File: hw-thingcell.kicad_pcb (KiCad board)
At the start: 2 copper layers, 32.5 x 67 mm, 99 parts, among them J1 Conn_01x02_Pin, J2 Conn_01x08_Pin, J3 USB4510-03-1-A, J4 Conn_01x08_Pin, J5 GSM_ANT, J6 GNSS_ANT, J7 SIM8060-6-0-14-00-A, Q1 PMBT3904235, Q2 PMBT3904235, Q3 PMBT3904235, U1 AP62301WU-7, U2 AP62301WU-7, U3 ESP32-S2-SOLO, U4 SIM868, U5 CH340C, Y1 32.768k

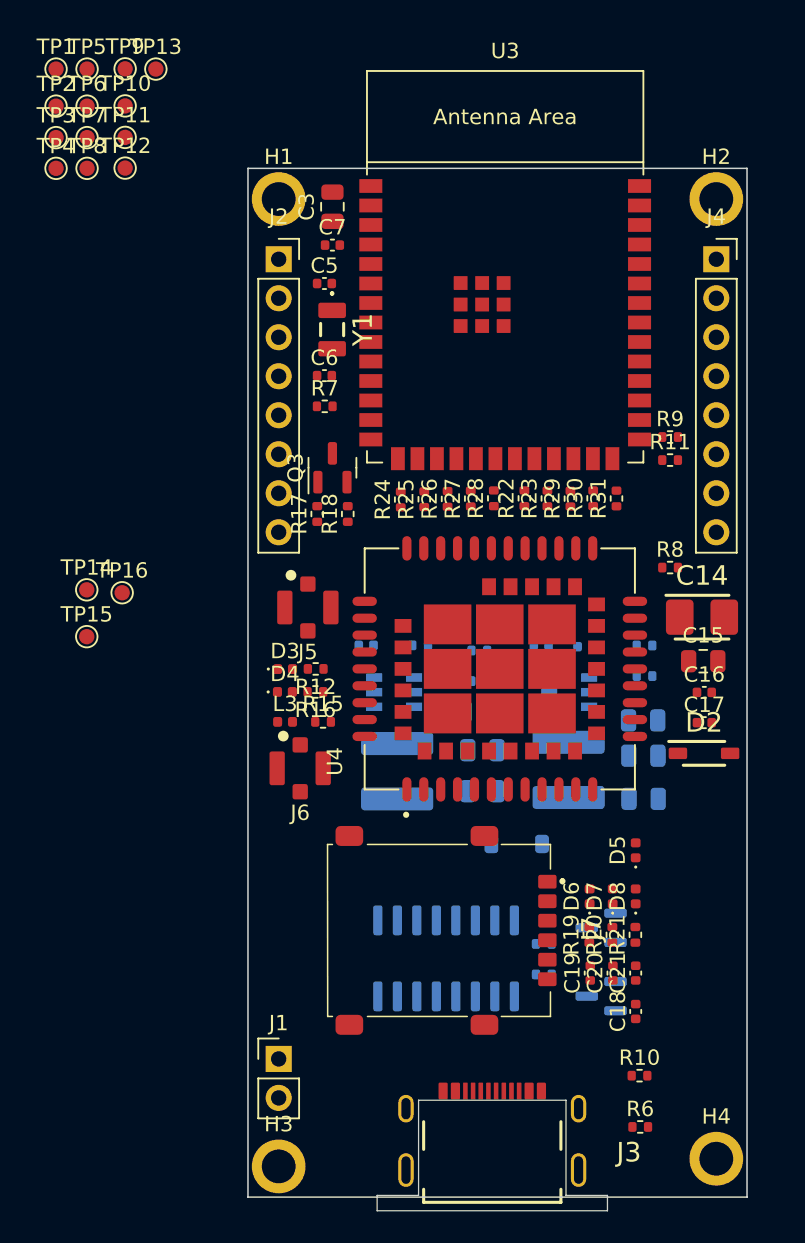
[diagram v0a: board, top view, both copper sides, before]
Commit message: First placement
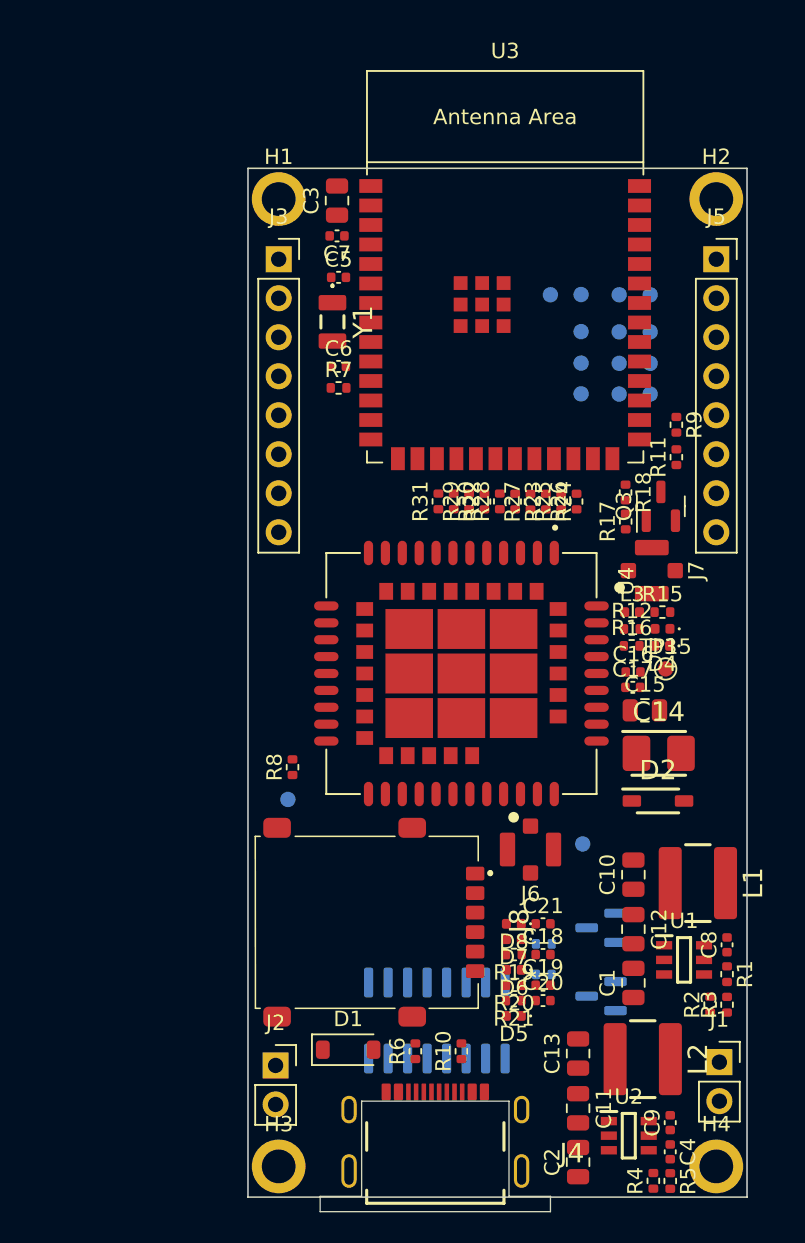
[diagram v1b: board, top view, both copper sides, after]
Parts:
- added J1: Conn_01x02_Pin, Connector_PinSocket_2.54mm:PinSocket_1x02_P2.54mm_Vertical, F.Cu at (151.7, 125.2)
- C1, C10, C11, C12, C13, C2, C4, C8, C9, D1, L1, L2, R1, R2, R3, R4, R5, U1, U2: moved to F.Cu
- J2: renamed from J1; footprint Connector_PinHeader_2.54mm:PinHeader_1x02_P2.54mm_Vertical -> Connector_PinSocket_2.54mm:PinSocket_1x02_P2.54mm_Vertical
- TP1, TP10, TP11, TP12, TP13, TP14, TP16, TP2, TP3, TP4, TP5, TP6, TP7, TP8, TP9: moved to B.Cu
- moved TP1 41.4 mm to (147.2, 75.2), turned to 180 degrees
- moved TP2 41.4 mm to (147.2, 77.7), turned to 180 degrees
- moved TP3 41.4 mm to (147.2, 79.7), turned to 180 degrees
- moved TP4 41.4 mm to (147.2, 81.7), turned to 180 degrees
- moved TP15 37.8 mm to (148.2, 99.6)
- moved TP5 37.6 mm to (145.2, 75.2), turned to 180 degrees
- moved TP6 37.6 mm to (145.2, 77.7), turned to 180 degrees
- moved TP7 37.6 mm to (145.2, 79.7), turned to 180 degrees
- moved TP8 37.6 mm to (145.2, 81.7), turned to 180 degrees
- moved R4 34.9 mm to (147.4, 132.9), turned to 90 degrees
- moved TP16 34.2 mm to (142.8, 111.0), turned to 180 degrees
- moved C4 33.4 mm to (148.5, 131.1), turned to -90 degrees
- moved TP10 33.1 mm to (142.7, 77.6), turned to 180 degrees
- moved TP11 33.1 mm to (142.7, 79.7), turned to 180 degrees
- moved TP12 33.1 mm to (142.7, 81.7), turned to 180 degrees
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- renumbered J2 to J3, J3 to J4, J4 to J5, J5 to J6, J6 to J7, J7 to J8

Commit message: Routed all components
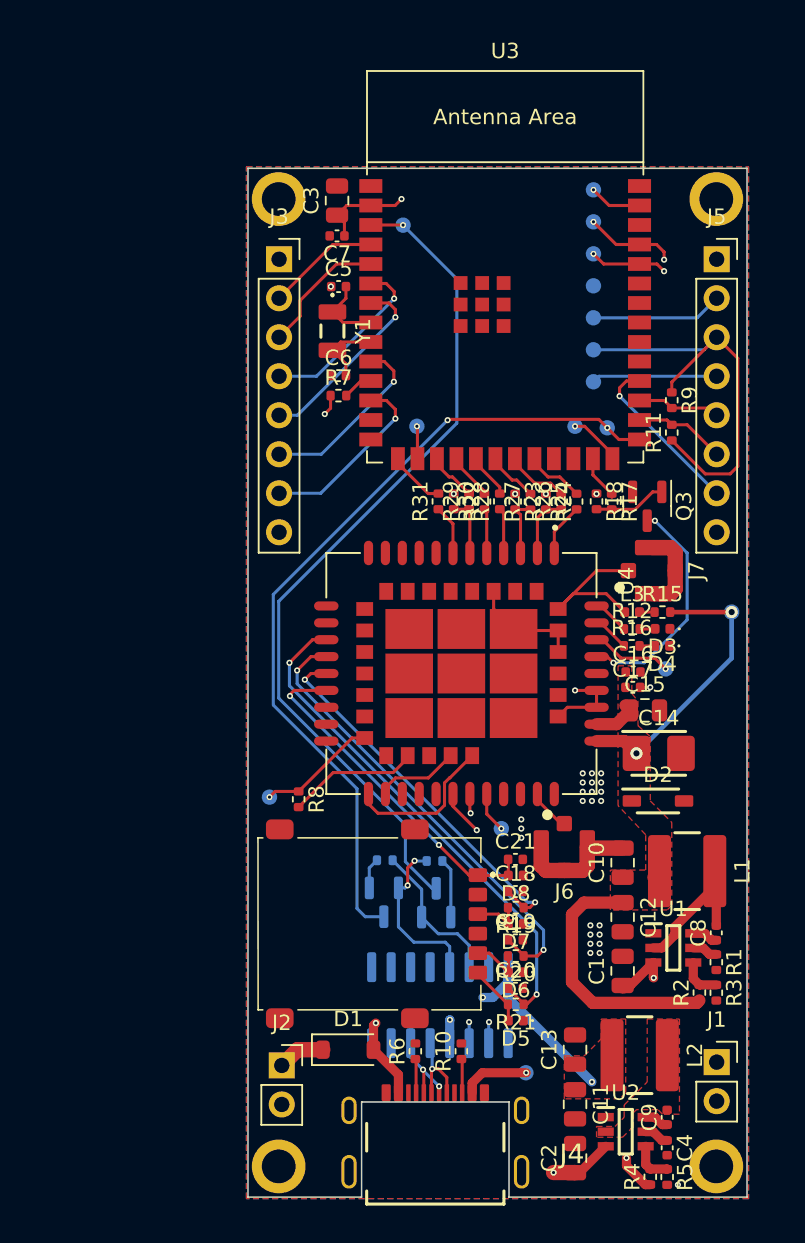
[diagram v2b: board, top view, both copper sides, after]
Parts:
- TP15: moved to B.Cu
- moved TP4 44.9 mm to (139.1, 125.9)
- moved TP3 17.0 mm to (152.5, 95.9)
- moved TP7 16.7 mm to (131.1, 70.7)
- moved Q2 15.4 mm to (129.8, 114.8), turned to -90 degrees
- moved TP8 13.3 mm to (132.0, 83.8)
- moved R14 12.7 mm to (129.9, 112.1), turned to 0 degrees
- moved Q1 10.9 mm to (133.3, 114.8), turned to 90 degrees
- moved TP11 9.24 mm to (143.5, 70.5)
- moved R13 8.93 mm to (133.2, 112.1)
- moved TP9 8.59 mm to (142.3, 83.8)
- moved TP13 7.39 mm to (143.5, 68.4)
- moved TP16 5.39 mm to (137.5, 110.0)
- moved TP10 5.13 mm to (143.5, 72.6)
- moved C21 4.56 mm to (138.4, 112.0)
- moved C18 4.48 mm to (138.4, 114.1)
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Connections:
- U3 pad 10: /D6/MOSI -> /D8
- U3 pad 12: /ESP_IO34 -> /D9/S_DET
- U3 pad 15: /ESP_RTS -> /ESP_IO34
- U3 pad 17: /PK_CTL -> /ESP_IO32
- U3 pad 18: /D1/SCL -> /ESP_IO33
- U3 pad 19: /D2/SDA -> /ESP_CTS
- U3 pad 20: /D3 -> /ESP_RTS
- U3 pad 21: /D4/SCK -> /ESP_TXD
- U3 pad 22: /D5/MISO -> /ESP_RXD
- U3 pad 24: /D7/SS -> unconnected-(U3-SPIIO4/GPIO33/FSPIHD-Pad24)
- U3 pad 25: /D8 -> /PK_CTL
- U3 pad 28: /D9/S_DET -> /D2/SDA
- U3 pad 29: unconnected-(U3-SPIIO7/GPIO36/FSPICLK-Pad29) -> /D1/SCL
- U3 pad 30: unconnected-(U3-SPIDQS/GPIO37/FSPIQ-Pad30) -> /D3
- U3 pad 38: /ESP_CTS -> unconnected-(U3-GPIO2/TOUCH2/ADC1_CH1-Pad38)
- U3 pad 4: /ESP_RXD -> /D4/SCK
- U3 pad 5: /ESP_TXD -> /D5/MISO
- U3 pad 6: /ESP_IO32 -> /D6/MOSI
- U3 pad 7: /ESP_IO33 -> /D7/SS
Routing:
- net /VIN: track 0.00 -> 105.8 mm, vias 0 -> 2
- net VBUS: track 0.00 -> 80.6 mm, vias 0 -> 1
- net /ESP_TX0: track 0.00 -> 67.4 mm, vias 0 -> 3
- net /ESP_RX0: track 0.00 -> 64.8 mm, vias 0 -> 3
- net /ESP_EN: track 0.00 -> 56.0 mm, vias 0 -> 1
- net +3V3: track 0.00 -> 54.1 mm, vias 0 -> 7
- net /ESP_IO0: track 0.00 -> 53.8 mm, vias 0 -> 2
- net +4V: track 0.00 -> 40.2 mm, vias 0 -> 2
- net /SIM_DATA: track 0.00 -> 33.9 mm, vias 0 -> 2
- net GND: track 0.00 -> 30.7 mm, vias 0 -> 32
- net /SIM_CLK: track 0.00 -> 30.0 mm, vias 0 -> 2
- net /SIM_RST: track 0.00 -> 24.9 mm, vias 0 -> 2
- net /SIM_VDD: track 0.00 -> 22.7 mm, vias 0 -> 2
- net /PWRKEY: track 0.00 -> 15.6 mm, vias 0 -> 2
- net /D9/S_DET: track 0.00 -> 12.7 mm, vias 0 -> 1
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- added copper zone on F.Cu, net +3V3
- added copper zone on In1.Cu, net +3V3
- added copper zone on F.Cu, net +4V
- added copper zone on B.Cu, net GND
- added copper zone on F.Cu, net GND
- added copper zone on In2.Cu, net GND
- added copper zone on F.Cu, net Net-(U2-SW)
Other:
- outline, holes or cut-outs redrawn
- copper layers 2 -> 4
